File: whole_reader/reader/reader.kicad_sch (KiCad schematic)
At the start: 59 parts, among them J1 Speaker+, J2 Speaker-, J3 Conn_02x05_Odd_Even, J4 USB_C_Receptacle_USB2.0_14P, J5 RFID RC522, J6 6P6C, SW1 SW_SPDT, SW2 SW_SPDT, U1 LM386, U2 STM32F103C8T6, U3 MCP16301Hx-xCH, U4 MAX3232, Y1 16MHz

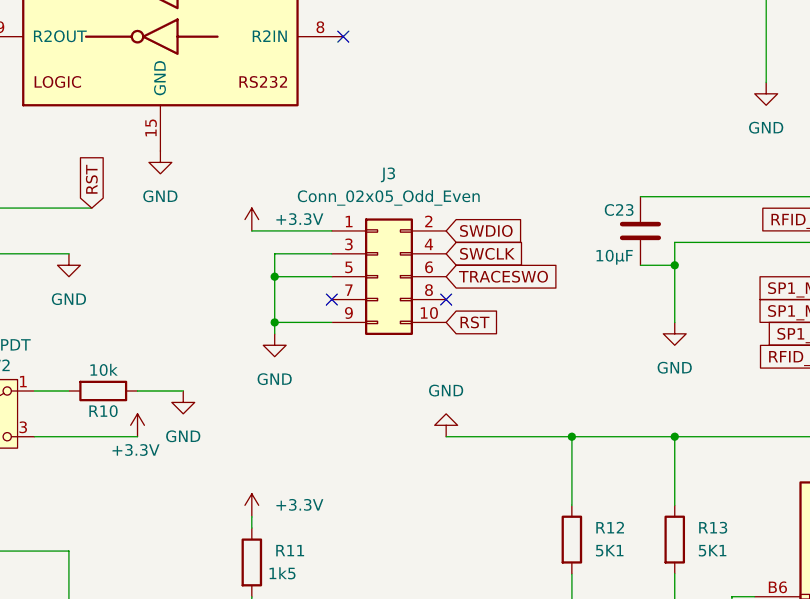
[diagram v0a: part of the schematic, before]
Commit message: trying adding solder pads
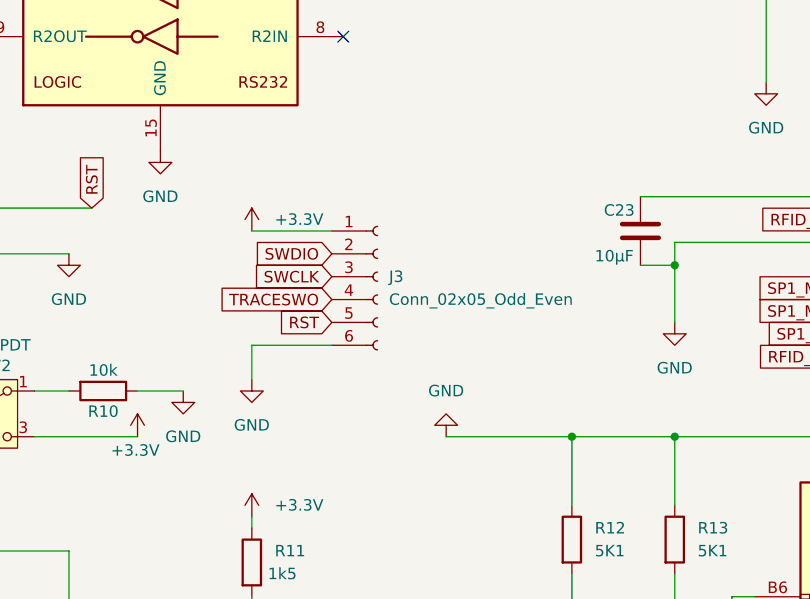
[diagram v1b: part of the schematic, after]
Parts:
- J3: footprint Connector_PinHeader_1.27mm:PinHeader_2x05_P1.27mm_Vertical_SMD -> Connector_PinHeader_2.54mm:PinHeader_1x06_P2.54mm_Vertical; symbol Connector_Generic:Conn_02x05_Odd_Even -> Connector:Conn_01x06_Socket
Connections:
- net GND: now also J3.6 (Pin_6); no longer J3.3 (Pin_3), J3.5 (Pin_5), J3.9 (Pin_9)
- net RST: now also J3.5 (Pin_5); no longer J3.10 (Pin_10)
- net SWCLK: now also J3.3 (Pin_3); no longer J3.4 (Pin_4)
- net TRACESWO: now also J3.4 (Pin_4); no longer J3.6 (Pin_6)
- no-connect marks 28 -> 26
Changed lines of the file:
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@@
 	)
 	(junction
-		(at 196.85 101.6)
-		(diameter 0)
-		(color 0 0 0 0)
-	)
-	(junction
 		(at 233.68 29.21)
 		(diameter 0)
@@
 		(color 0 0 0 0)
 	)
-	(junction
-		(at 196.85 106.68)
-		(diameter 0)
-		(color 0 0 0 0)
-	)
 	(no_connect
 		(at 90.17 130.81)
@@
 	)
 	(no_connect
-		(at 203.2 104.14)
-	)
-	(no_connect
 		(at 90.17 125.73)
 	)
@@
 	)
 	(no_connect
-		(at 215.9 104.14)
-	)
-	(no_connect
 		(at 204.47 74.93)
 	)
@@
 	(wire
 		(pts
-			(xy 196.85 101.6) (xy 203.2 101.6)
-		)
-		(stroke
-			(width 0)
-			(type default)
-		)
-	)
-	(wire
-		(pts
 			(xy 48.26 26.67) (xy 48.26 31.75)
 		)
@@
 	(wire
 		(pts
-			(xy 196.85 106.68) (xy 196.85 107.95)
-		)
-		(stroke
-			(width 0)
-			(type default)
-		)
-	)
-	(wire
-		(pts
 			(xy 264.16 50.8) (xy 232.41 50.8)
 		)
@@
 	(wire
 		(pts
-			(xy 196.85 106.68) (xy 203.2 106.68)
-		)
-		(stroke
-			(width 0)
-			(type default)
-		)
-	)
-	(wire
-		(pts
 			(xy 238.76 45.72) (xy 233.68 45.72)
 		)
@@
 	(wire
 		(pts
-			(xy 229.87 119.38) (xy 215.9 119.38)
+			(xy 194.31 109.22) (xy 194.31 113.03)
 		)
 		(stroke
@@
 	(wire
 		(pts
-			(xy 80.01 83.82) (xy 80.01 85.09)
+			(xy 229.87 119.38) (xy 215.9 119.38)
 		)
 		(stroke
@@
 	(wire
 		(pts
-			(xy 35.56 31.75) (xy 35.56 33.02)
+			(xy 80.01 83.82) (xy 80.01 85.09)
 		)
 		(stroke
@@
 	(wire
 		(pts
-			(xy 154.94 153.67) (xy 147.32 153.67)
+			(xy 35.56 31.75) (xy 35.56 33.02)
 		)
 		(stroke
@@
 	(wire
 		(pts
-			(xy 165.1 187.96) (xy 165.1 186.69)
+			(xy 154.94 153.67) (xy 147.32 153.67)
 		)
 		(stroke
@@
 	(wire
 		(pts
-			(xy 241.3 100.33) (xy 241.3 106.68)
+			(xy 165.1 187.96) (xy 165.1 186.69)
 		)
 		(stroke
@@
 	(wire
 		(pts
-			(xy 90.17 86.36) (xy 80.01 86.36)
+			(xy 241.3 100.33) (xy 241.3 106.68)
 		)
 		(stroke
@@
 	(wire
 		(pts
-			(xy 130.81 26.67) (xy 130.81 35.56)
+			(xy 90.17 86.36) (xy 80.01 86.36)
 		)
 		(stroke
@@
 	(wire
 		(pts
-			(xy 196.85 99.06) (xy 196.85 101.6)
+			(xy 130.81 26.67) (xy 130.81 35.56)
 		)
 		(stroke
@@
 	(wire
 		(pts
-			(xy 203.2 99.06) (xy 196.85 99.06)
-		)
-		(stroke
-			(width 0)
-			(type default)
-		)
-	)
-	(wire
-		(pts
 			(xy 68.58 60.96) (xy 68.58 67.31)
 		)
@@
 	(wire
 		(pts
+			(xy 203.2 109.22) (xy 194.31 109.22)
+		)
+		(stroke
+			(width 0)
+			(type default)
+		)
+	)
+	(wire
+		(pts
 			(xy 165.1 147.32) (xy 173.99 147.32)
 		)
@@
 	(wire
 		(pts
-			(xy 196.85 101.6) (xy 196.85 106.68)
-		)
-		(stroke
-			(width 0)
-			(type default)
-		)
-	)
-	(wire
-		(pts
 			(xy 257.81 67.31) (xy 257.81 72.39)
 		)
@@
 	(global_label "TRACESWO"
 		(shape input)
-		(at 215.9 101.6 0)
+		(at 203.2 104.14 180)
 		(fields_autoplaced yes)
 		(effects
@@
 				(size 1.27 1.27)
 			)
-			(justify left)
+			(justify right)
 		)
 		(property "Intersheetrefs" "${INTERSHEET_REFS}"
-			(at 228.6218 101.6 0)
+			(at 190.4782 104.14 0)
 			(effects
 				(font
 					(size 1.27 1.27)
 				)
-				(justify left)
+				(justify right)
 				(hide yes)
 			)
@@
 	(global_label "SWCLK"
 		(shape input)
-		(at 215.9 99.06 0)
+		(at 203.2 101.6 180)
 		(fields_autoplaced yes)
 		(effects
@@
 				(size 1.27 1.27)
 			)
-			(justify left)
+			(justify right)
 		)
 		(property "Intersheetrefs" "${INTERSHEET_REFS}"
-			(at 225.1142 99.06 0)
+			(at 193.9858 101.6 0)
 			(effects
 				(font
 					(size 1.27 1.27)
 				)
-				(justify left)
+				(justify right)
 				(hide yes)
 			)
@@
 	(global_label "SWDIO"
 		(shape input)
-		(at 215.9 96.52 0)
+		(at 203.2 99.06 180)
 		(fields_autoplaced yes)
 		(effects
@@
 				(size 1.27 1.27)
 			)
-			(justify left)
+			(justify right)
 		)
 		(property "Intersheetrefs" "${INTERSHEET_REFS}"
-			(at 224.7514 96.52 0)
+			(at 194.3486 99.06 0)
 			(effects
 				(font
 					(size 1.27 1.27)
 				)
-				(justify left)
+				(justify right)
 				(hide yes)
 			)
@@
 	(global_label "RST"
 		(shape input)
-		(at 215.9 106.68 0)
+		(at 203.2 106.68 180)
 		(fields_autoplaced yes)
 		(effects
@@
 				(size 1.27 1.27)
 			)
-			(justify left)
+			(justify right)
 		)
 		(property "Intersheetrefs" "${INTERSHEET_REFS}"
-			(at 222.3323 106.68 0)
+			(at 196.7677 106.68 0)
 			(effects
 				(font
 					(size 1.27 1.27)
 				)
-				(justify left)
+				(justify right)
 				(hide yes)
 			)
@@
 	)
 	(symbol
-		(lib_id "Connector_Generic:Conn_02x05_Odd_Even")
+		(lib_id "Connector:Conn_01x06_Socket")
 		(at 208.28 101.6 0)
 		(unit 1)
@@
 		(fields_autoplaced yes)
 		(property "Reference" "J3"
-			(at 209.55 90.17 0)
+			(at 209.55 101.5999 0)
 			(effects
 				(font
 					(size 1.27 1.27)
 				)
+				(justify left)
 			)
 		)
 		(property "Value" "Conn_02x05_Odd_Even"
-			(at 209.55 92.71 0)
+			(at 209.55 104.1399 0)
 			(effects
 				(font
 					(size 1.27 1.27)
 				)
+				(justify left)
 			)
 		)
-		(property "Footprint" "Connector_PinHeader_1.27mm:PinHeader_2x05_P1.27mm_Vertical_SMD"
+		(property "Footprint" "Connector_PinHeader_2.54mm:PinHeader_1x06_P2.54mm_Vertical"
 			(at 208.28 101.6 0)
 			(effects
@@
 			)
 		)
-		(property "Description" "Generic connector, double row, 02x05, odd/even pin numbering scheme (row 1 odd numbers, row 2 even numbers), script generated (kicad-library-utils/schlib/autogen/connector/)"
+		(property "Description" "Generic connector, single row, 01x06, script generated"
 			(at 208.28 101.6 0)
 			(effects
@@
 		(pin "5"
 		)
-		(pin "7"
-		)
-		(pin "10"
-		)
-		(pin "8"
-		)
 		(pin "3"
 		)
-		(pin "9"
-		)
 		(instances
 			(project "reader"
@@
 	)
 	(symbol
-		(lib_id "power:GND")
-		(at 196.85 107.95 0)
-		(unit 1)
-		(exclude_from_sim no)
-		(in_bom yes)
-		(on_board yes)
-		(dnp no)
-		(fields_autoplaced yes)
-		(property "Reference" "#PWR033"
-			(at 196.85 114.3 0)
-			(effects
-				(font
-					(size 1.27 1.27)
-				)
-				(hide yes)
-			)
-		)
-		(property "Value" "GND"
-			(at 196.85 113.03 0)
-			(effects
-				(font
-					(size 1.27 1.27)
-				)
-			)
-		)
-		(property "Footprint" ""
-			(at 196.85 107.95 0)
-			(effects
-				(font
-					(size 1.27 1.27)
-				)
-				(hide yes)
-			)
-		)
-		(property "Datasheet" ""
-			(at 196.85 107.95 0)
-			(effects
-				(font
-					(size 1.27 1.27)
-				)
-				(hide yes)
-			)
-		)
-		(property "Description" "Power symbol creates a global label with name \"GND\" , ground"
-			(at 196.85 107.95 0)
-			(effects
-				(font
-					(size 1.27 1.27)
-				)
-				(hide yes)
-			)
-		)
-		(pin "1"
-		)
-		(instances
-			(project "reader"
-				(path "/6275a1a7-d424-4390-b849-2e49b1a9780b"
-					(reference "#PWR033")
-					(unit 1)
-				)
-			)
-		)
-	)
-	(symbol
 		(lib_id "Connector:Conn_01x01_Socket")
 		(at 83.82 55.88 90)
@@
 					(unit 1)
 				)
+			)
+		)
+	)
+	(symbol
+		(lib_id "power:GND")
+		(at 194.31 113.03 0)
+		(unit 1)
+		(exclude_from_sim no)
+		(in_bom yes)
+		(on_board yes)
+		(dnp no)
+		(fields_autoplaced yes)
+		(property "Reference" "#PWR033"
+			(at 194.31 119.38 0)
+			(effects
+				(font
+					(size 1.27 1.27)
+				)
+				(hide yes)
+			)
+		)
+		(property "Value" "GND"
+			(at 194.31 118.11 0)
+			(effects
+				(font
+					(size 1.27 1.27)
+				)
+			)
+		)
+		(property "Footprint" ""
+			(at 194.31 113.03 0)
+			(effects
+				(font
+					(size 1.27 1.27)
+				)
+				(hide yes)
+			)
+		)
+		(property "Datasheet" ""
+			(at 194.31 113.03 0)
+			(effects
+				(font
+					(size 1.27 1.27)
+				)
+				(hide yes)
+			)
+		)
+		(property "Description" "Power symbol creates a global label with name \"GND\" , ground"
+			(at 194.31 113.03 0)
+			(effects
+				(font
+					(size 1.27 1.27)
+				)
+				(hide yes)
+			)
+		)
+		(pin "1"
+		)
+		(instances
+			(project ""
+				(path "/6275a1a7-d424-4390-b849-2e49b1a9780b"
+					(reference "#PWR033")
+					(unit 1)
+				)
